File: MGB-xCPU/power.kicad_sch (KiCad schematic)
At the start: 29 parts, among them P4 DC 3V, Q2 2SC4081, SW1 SP3T, U5 DC/DC

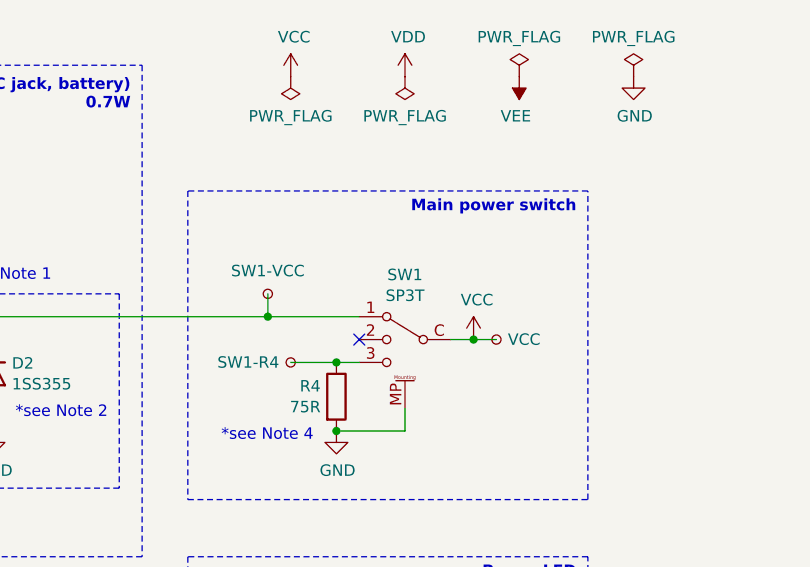
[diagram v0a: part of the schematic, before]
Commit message: Tidy up switch symbols
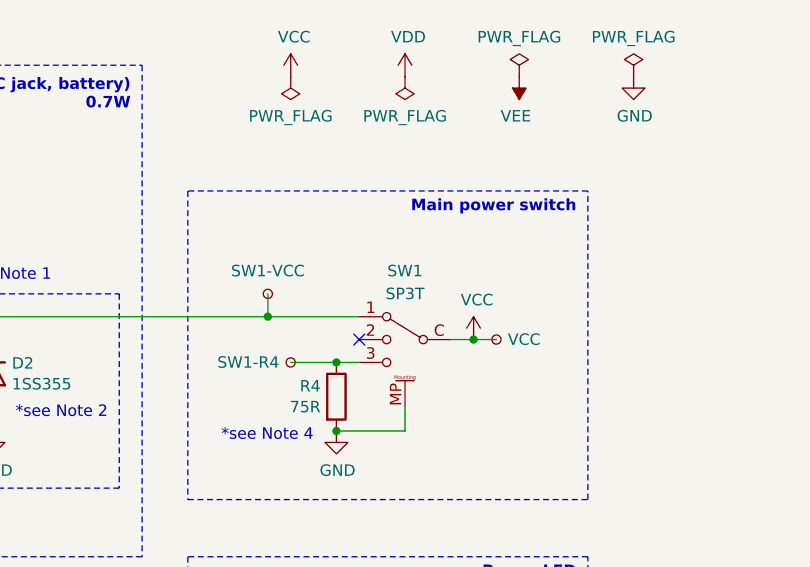
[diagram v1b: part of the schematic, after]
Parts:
- SW1: symbol Gekkio_Switch:GameBoy_SW_SP3T -> Gekkio_Switch:GameBoy_SW_SP3T_MGB
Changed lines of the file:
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@@
     )
   )
-  (symbol (lib_id "Gekkio_Switch:GameBoy_SW_SP3T") (at 165.1 54.61 0) (mirror y) (unit 1)
-    (in_bom yes) (on_board yes) (dnp no)
-    (property "Reference" "SW1" (at 165.1 47.4218 0)
+  (symbol (lib_id "Gekkio_Switch:GameBoy_SW_SP3T_MGB") (at 165.1 54.61 0) (mirror y) (unit 1)
+    (in_bom yes) (on_board yes) (dnp no) (fields_autoplaced)
+    (property "Reference" "SW1" (at 165.1 46.99 0)
       (effects (font (size 1.27 1.27)))
     )
-    (property "Value" "SP3T" (at 165.1 49.7332 0)
+    (property "Value" "SP3T" (at 165.1 49.53 0)
       (effects (font (size 1.27 1.27)))
     )
